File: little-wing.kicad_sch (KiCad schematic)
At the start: 72 parts, among them IC1 AP7335-WG-7, J1 nice!view, J2 Battery, J3 trackball, J4 trackball, SW1 Power, SW2 Reset, U1 nice!nano v2, U2 PMW3610

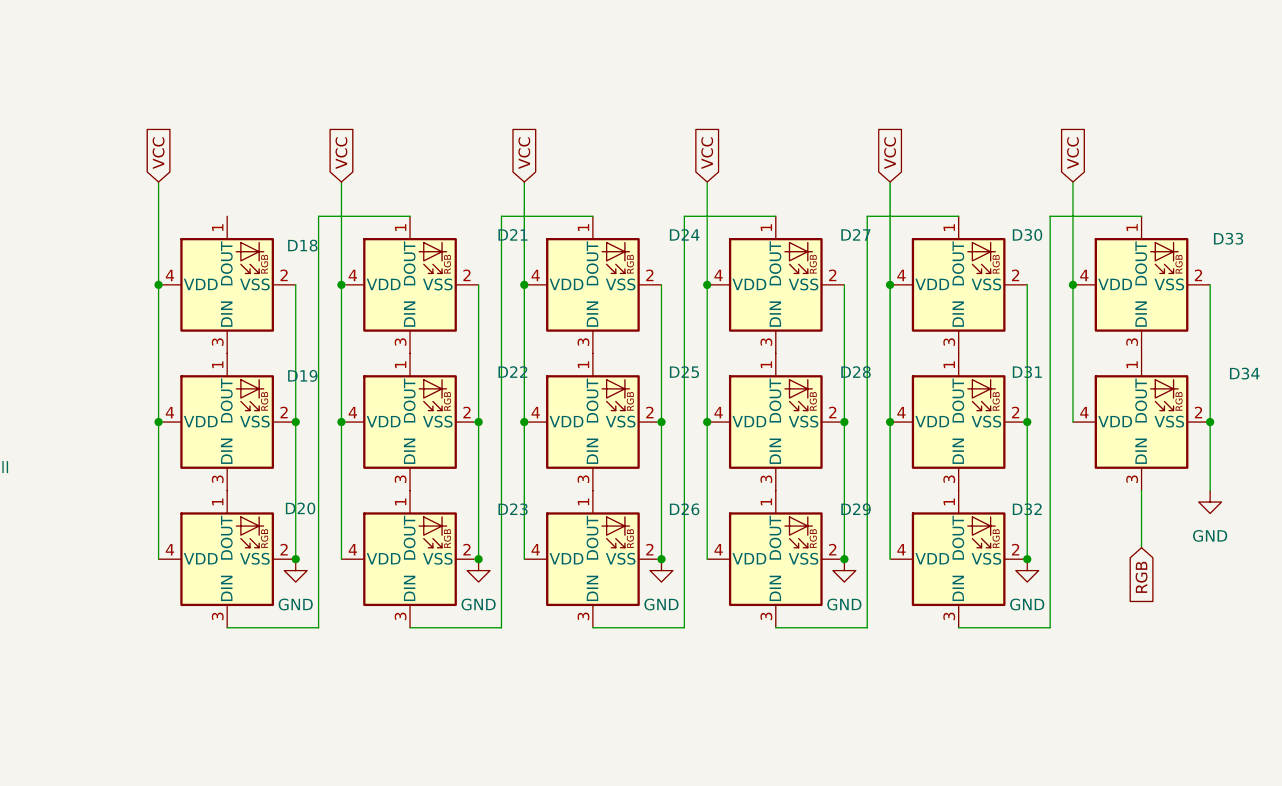
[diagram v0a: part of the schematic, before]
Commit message: Making a column work
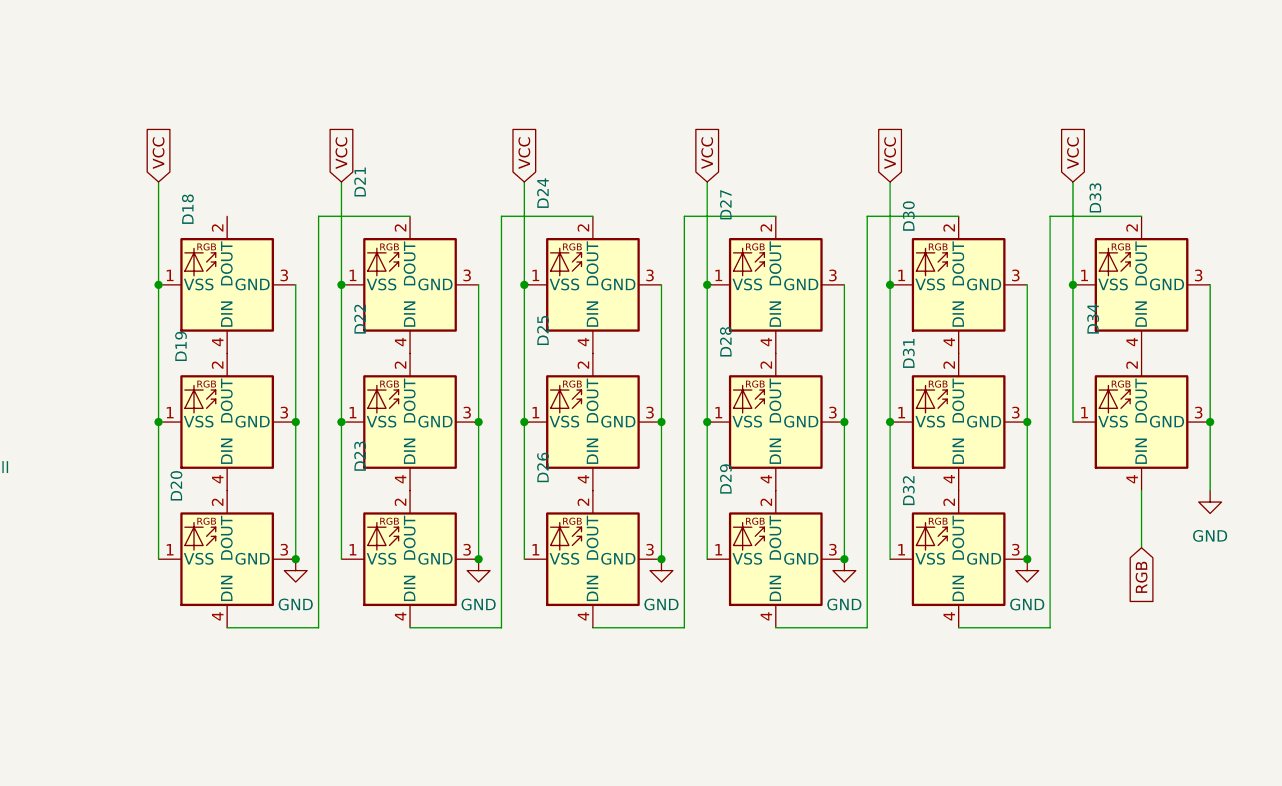
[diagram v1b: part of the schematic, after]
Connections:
- net GND: now also D18.3 (GND), D19.3 (GND), D20.3 (GND), D21.3 (GND), D22.3 (GND), D23.3 (GND), D24.3 (GND), D25.3 (GND), D26.3 (GND), D27.3 (GND), D28.3 (GND), D29.3 (GND), D30.3 (GND), D31.3 (GND), D32.3 (GND), D33.3 (GND), D34.3 (GND); no longer D18.2 (VSS), D19.2 (VSS), D20.2 (VSS), D21.2 (VSS), D22.2 (VSS), D23.2 (VSS), D24.2 (VSS), D25.2 (VSS), D26.2 (VSS), D27.2 (VSS), D28.2 (VSS), D29.2 (VSS), D30.2 (VSS), D31.2 (VSS), D32.2 (VSS), D33.2 (VSS), D34.2 (VSS)
- net RGB: now also D34.4 (DIN); no longer D34.3 (DIN)
- net VCC: now also D18.1 (VSS), D19.1 (VSS), D20.1 (VSS), D21.1 (VSS), D22.1 (VSS), D23.1 (VSS), D24.1 (VSS), D25.1 (VSS), D26.1 (VSS), D27.1 (VSS), D28.1 (VSS), D29.1 (VSS), D30.1 (VSS), D31.1 (VSS), D32.1 (VSS), D33.1 (VSS), D34.1 (VSS); no longer D18.4 (VDD), D19.4 (VDD), D20.4 (VDD), D21.4 (VDD), D22.4 (VDD), D23.4 (VDD), D24.4 (VDD), D25.4 (VDD), D26.4 (VDD), D27.4 (VDD), D28.4 (VDD), D29.4 (VDD), D30.4 (VDD), D31.4 (VDD), D32.4 (VDD), D33.4 (VDD), D34.4 (VDD)
- new net: D31.4 (DIN), D32.2 (DOUT)
- new net: D32.4 (DIN), D33.2 (DOUT)
- new net: D28.4 (DIN), D29.2 (DOUT)
- new net: D29.4 (DIN), D30.2 (DOUT)
- new net: D19.4 (DIN), D20.2 (DOUT)
- new net: D20.4 (DIN), D21.2 (DOUT)
- new net: D23.4 (DIN), D24.2 (DOUT)
- new net: D24.4 (DIN), D25.2 (DOUT)
- new net: D22.4 (DIN), D23.2 (DOUT)
- new net: D25.4 (DIN), D26.2 (DOUT)
- new net: D21.4 (DIN), D22.2 (DOUT)
- new net: D30.4 (DIN), D31.2 (DOUT)
- new net: D18.4 (DIN), D19.2 (DOUT)
- new net: D27.4 (DIN), D28.2 (DOUT)
- new net: D26.4 (DIN), D27.2 (DOUT)
- new net: D33.4 (DIN), D34.2 (DOUT)
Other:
- moved on the sheet: D18, D19, D20, D21, D22, D23, D24, D25, D26, D27, D28, D29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
